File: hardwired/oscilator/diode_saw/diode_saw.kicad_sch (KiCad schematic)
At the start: 21 parts, among them Q1 PNP, Q2 NPN, U1 ${SIM.PARAMS}, U2 ${SIM.PARAMS}

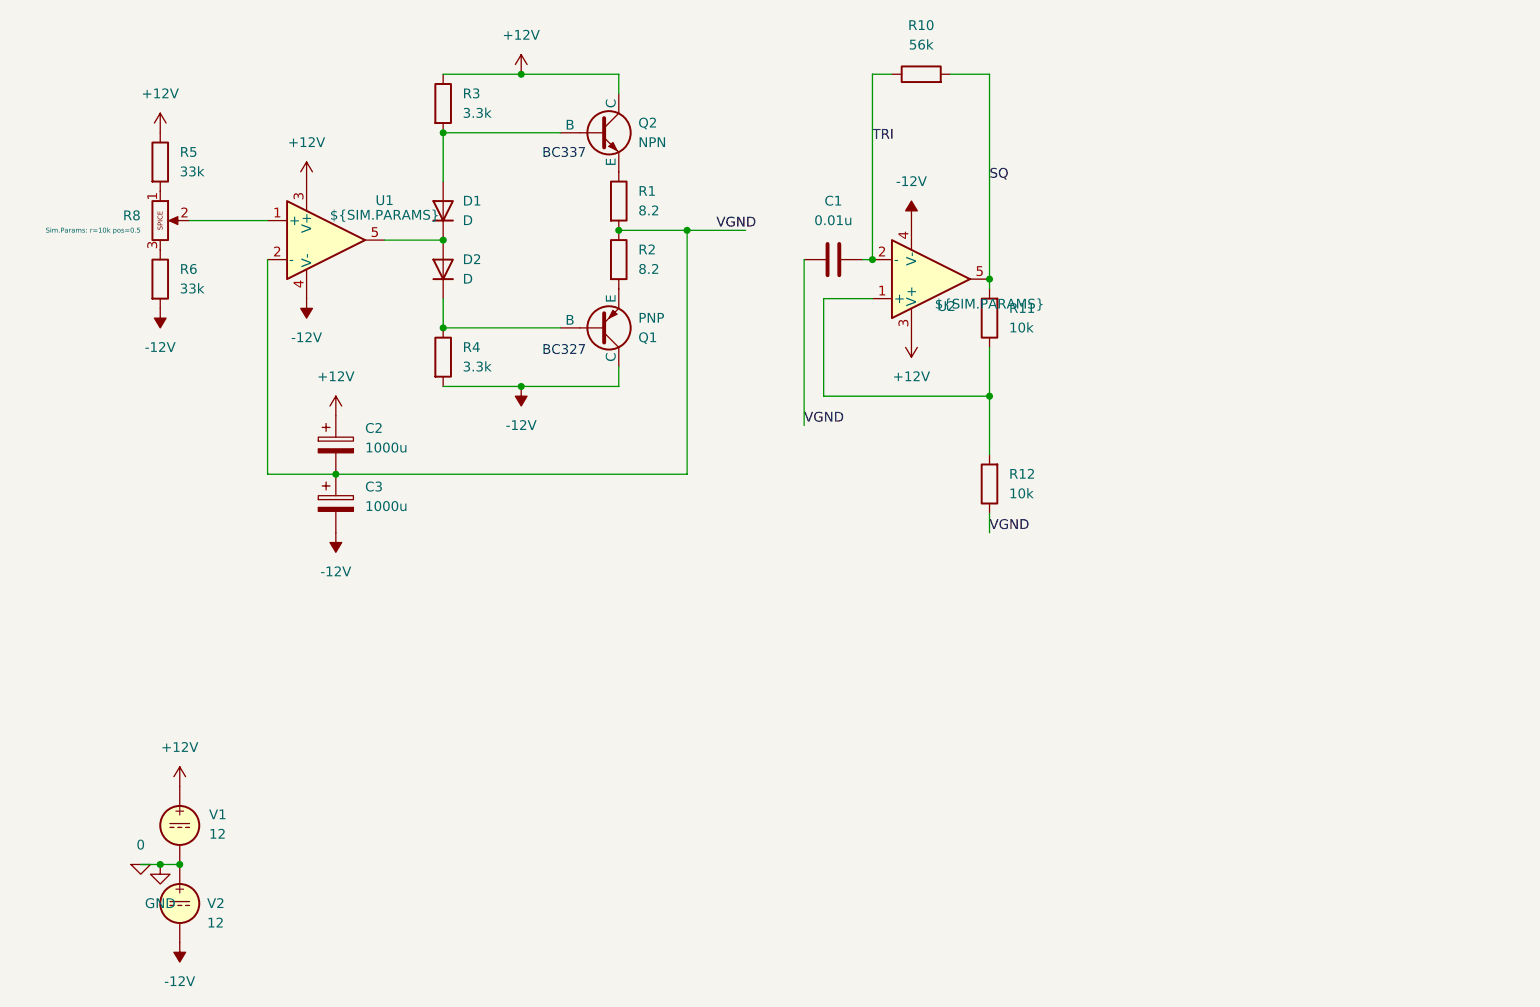
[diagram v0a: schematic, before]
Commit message: Massive dump of circuits and code
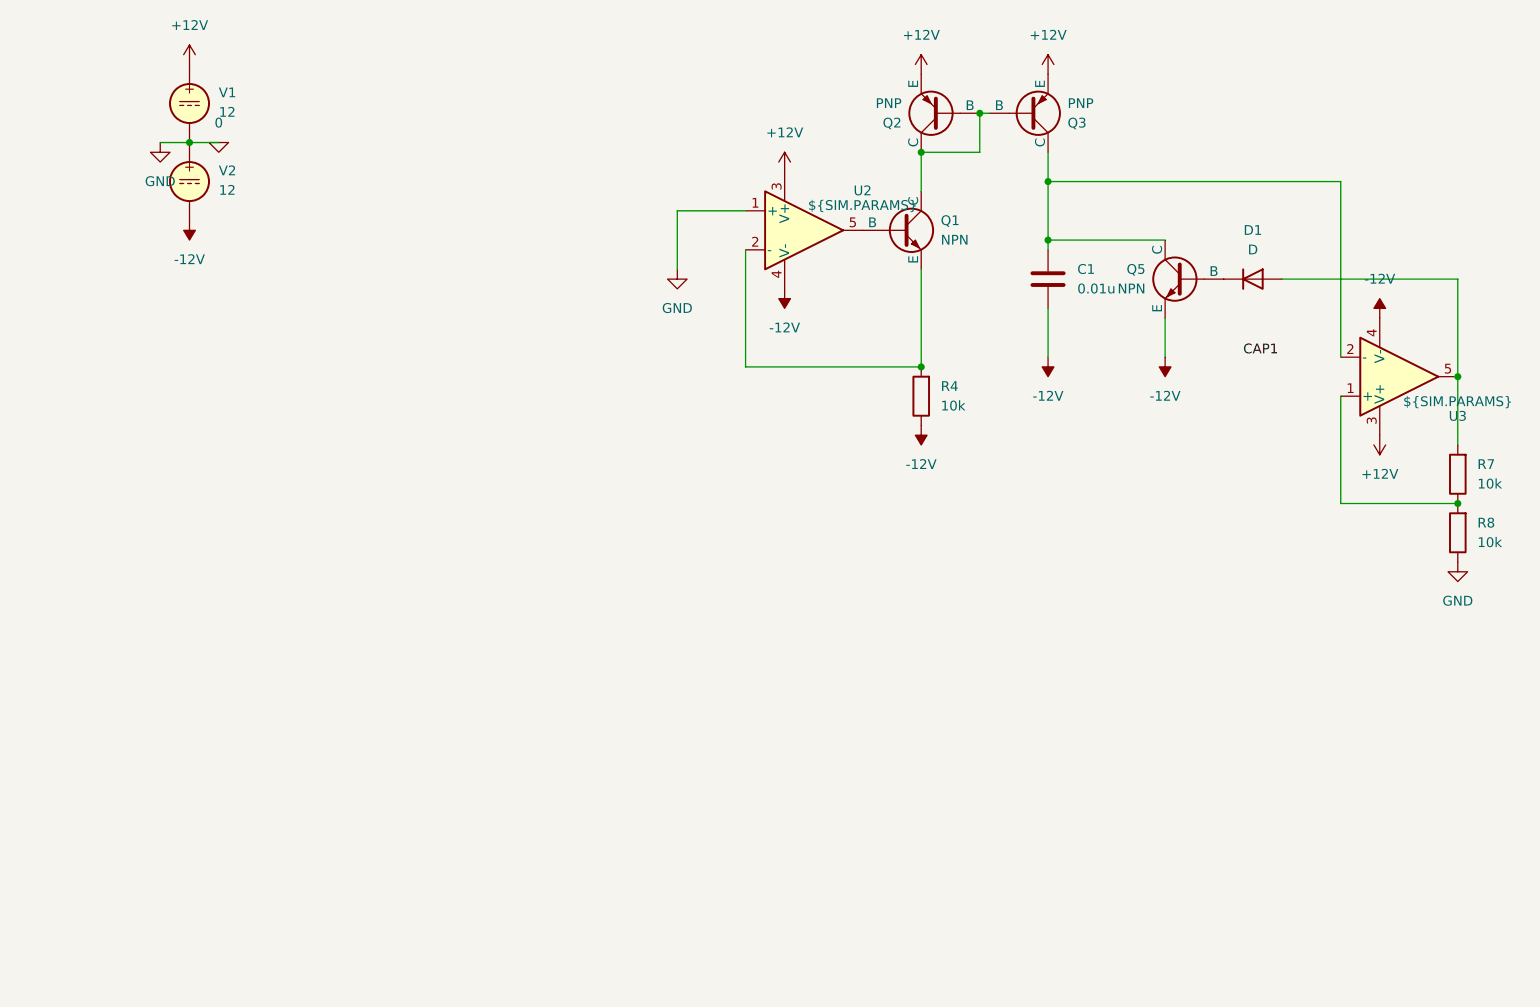
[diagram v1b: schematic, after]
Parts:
- removed C2, C3: 1000u, Connector_PinSocket_2.54mm:PinSocket_1x02_P2.54mm_Vertical, symbol Device:C_Polarized
- removed D2: D, Diode_THT:D_A-405_P7.62mm_Horizontal, symbol Device:D
- removed Q1: PNP, Connector_PinSocket_2.54mm:PinSocket_1x03_P2.54mm_Vertical, symbol Simulation_SPICE:PNP
- removed Q2: NPN, Connector_PinSocket_2.54mm:PinSocket_1x03_P2.54mm_Vertical, symbol Simulation_SPICE:NPN
- removed R1, R2: 8.2, Resistor_THT:R_Axial_DIN0309_L9.0mm_D3.2mm_P15.24mm_Horizontal, symbol Device:R
- removed R10: 56k, Resistor_THT:R_Axial_DIN0411_L9.9mm_D3.6mm_P15.24mm_Horizontal, symbol Device:R
- removed R11, R12: 10k, Resistor_THT:R_Axial_DIN0411_L9.9mm_D3.6mm_P15.24mm_Horizontal, symbol Device:R
- removed R3: 3.3k, Resistor_THT:R_Axial_DIN0309_L9.0mm_D3.2mm_P15.24mm_Horizontal, symbol Device:R
- removed R5, R6: 33k, Resistor_THT:R_Axial_DIN0309_L9.0mm_D3.2mm_P15.24mm_Horizontal, symbol Device:R
- removed R8: Potentiometer, Connector_PinHeader_2.54mm:PinHeader_1x03_P2.54mm_Horizontal, symbol Simulation_SPICE:Potentiometer
- removed U1: ${SIM.PARAMS}, Package_DIP:DIP-8_W7.62mm, symbol Simulation_SPICE:OPAMP
- added Q1, Q5: NPN, symbol Simulation_SPICE:NPN
- added Q2, Q3: PNP, symbol Simulation_SPICE:PNP
- added R7, R8: 10k, symbol Device:R
- added U3: ${SIM.PARAMS}, symbol Simulation_SPICE:OPAMP
- D1: footprint Diode_THT:D_A-405_P7.62mm_Horizontal -> (none)
- R4: value 3.3k -> 10k; footprint Resistor_THT:R_Axial_DIN0309_L9.0mm_D3.2mm_P15.24mm_Horizontal -> (none)
- U2: footprint Package_DIP:DIP-8_W7.62mm -> (none)
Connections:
- net +12V: now also Q2.3 (E), Q3.3 (E), U3.3 (V+)
- net -12V: now also C1.2, R4.1, Q5.3 (E), U3.4 (V-); no longer R4.2
- net 0: now also U2.1 (+), R8.1
- net at D1.1 (K): now also Q5.2 (B)
- net at D1.2 (A): now also R7.2, U3.5
- net SQ: no longer names the net of U2.5
- net SQ: now also Q1.2 (B)
- net TRI: no longer names the net of U2.2 (-)
- net TRI: now also R4.2, Q1.3 (E); no longer C1.2
- net VGND: no longer names the net of C1.1
- net VGND: now also Q3.1 (C), Q5.1 (C), U3.2 (-)
- new net: Q1.1 (C), Q2.1 (C), Q2.2 (B), Q3.2 (B)
- new net: R7.1, R8.2, U3.1 (+)
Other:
- note removed: "BC327"
- note removed: "BC337"
